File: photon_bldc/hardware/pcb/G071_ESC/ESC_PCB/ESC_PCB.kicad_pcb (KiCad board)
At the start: 4 copper layers, 36 x 16 mm, 69 parts, among them J2 Plus, J3 Minus, Q1 NMOS, Q2 NMOS, Q3 NMOS, Q4 NMOS, Q5 NMOS, Q6 NMOS, U1 STM32G071GBUx, U4 L78L06_SOT89

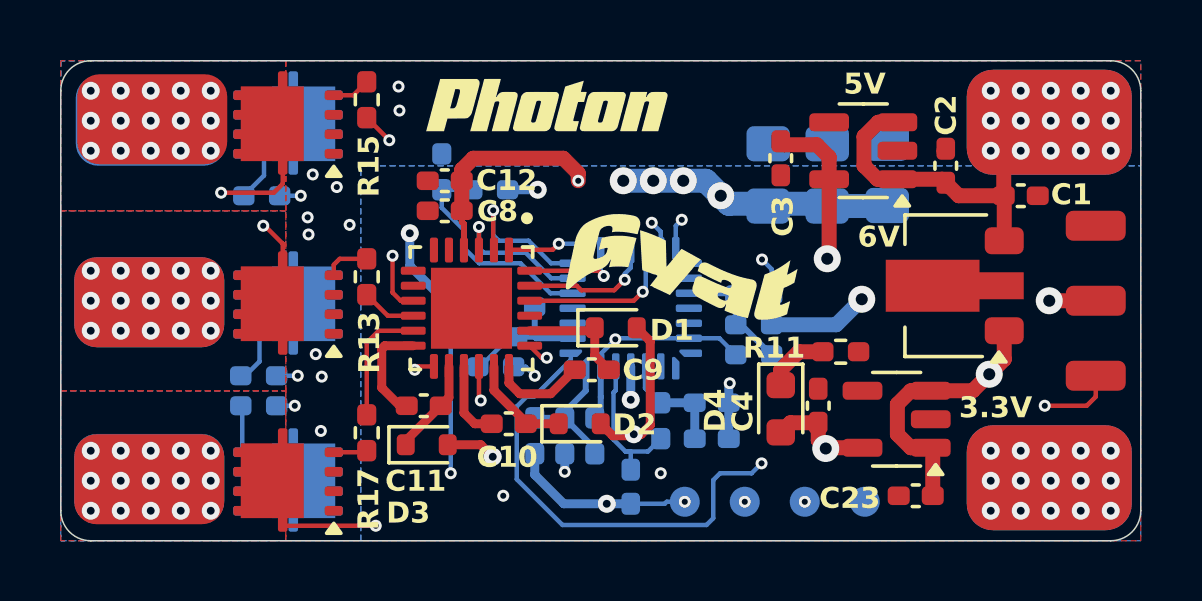
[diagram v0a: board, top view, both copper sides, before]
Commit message: 22.04.2025
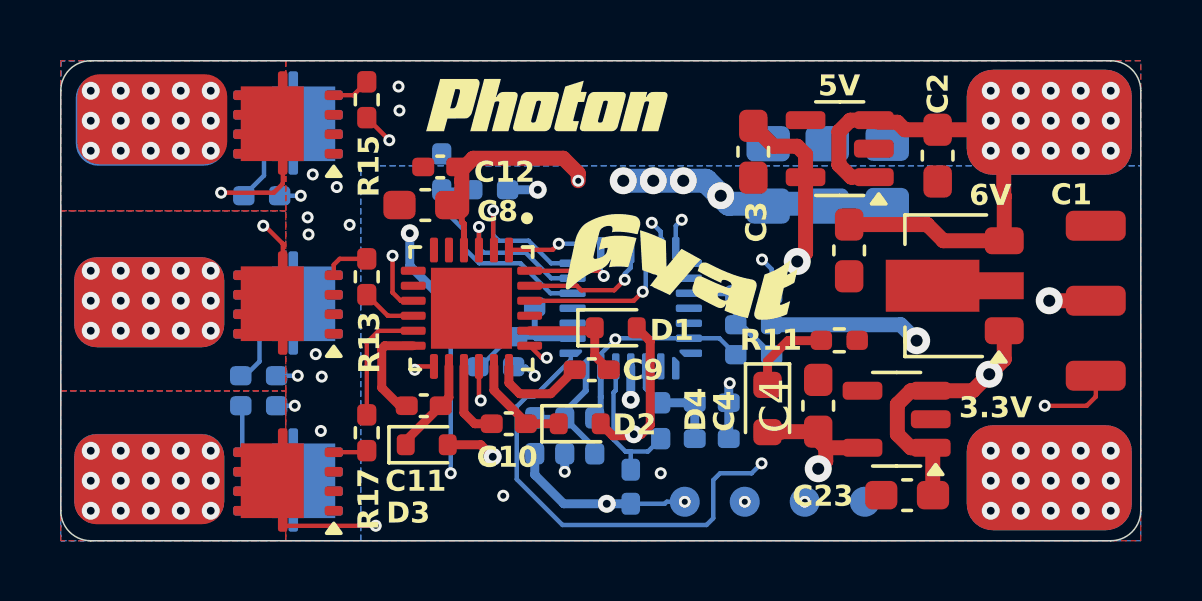
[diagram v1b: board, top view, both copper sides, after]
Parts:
- C1, C2, C23, C3, C4, C8: footprint Capacitor_SMD:C_0402_1005Metric_Pad0.74x0.62mm_HandSolder -> Capacitor_SMD:C_0603_1608Metric_Pad1.08x0.95mm_HandSolder
- moved C1 6.00 mm to (97.3, 50.3), turned to -90 degrees
- moved C3 0.94 mm to (94.1, 47.0)
- moved U2 0.79 mm to (97.0, 46.9)
- moved C8 0.67 mm to (83.2, 48.8)
- moved C12 0.48 mm to (83.7, 47.5)
- moved D4 0.44 mm to (94.6, 55.6)
- moved C2 0.43 mm to (100.2, 47.2), turned to -90 degrees
- moved R11 0.38 mm to (97.0, 53.3)
- moved C23 0.29 mm to (99.2, 58.5)
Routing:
- net VDC: track 12.0 -> 17.2 mm
- net +5V: track 15.9 -> 17.5 mm
- net GND: track 26.8 -> 28.4 mm
- net Net-(D4-K): track 2.16 -> 2.87 mm
